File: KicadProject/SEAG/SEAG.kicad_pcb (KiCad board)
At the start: 4 copper layers, 99.6 x 63 mm, 64 parts, among them J1 Screw_Terminal_01x02, J10 Screw_Terminal_01x02, J11 Screw_Terminal_01x02, J12 Screw_Terminal_01x02, J13 Conn_01x03_Pin, J2 Conn_01x06_Pin, J3 Screw_Terminal_01x02, J4 Screw_Terminal_01x02, J5 Screw_Terminal_01x02, J6 Screw_Terminal_01x02, J7 Screw_Terminal_01x02, J8 Screw_Terminal_01x02, J9 Screw_Terminal_01x02, U1 STM32F722RCTx, X1 XO32, Y1 Crystal_GND24

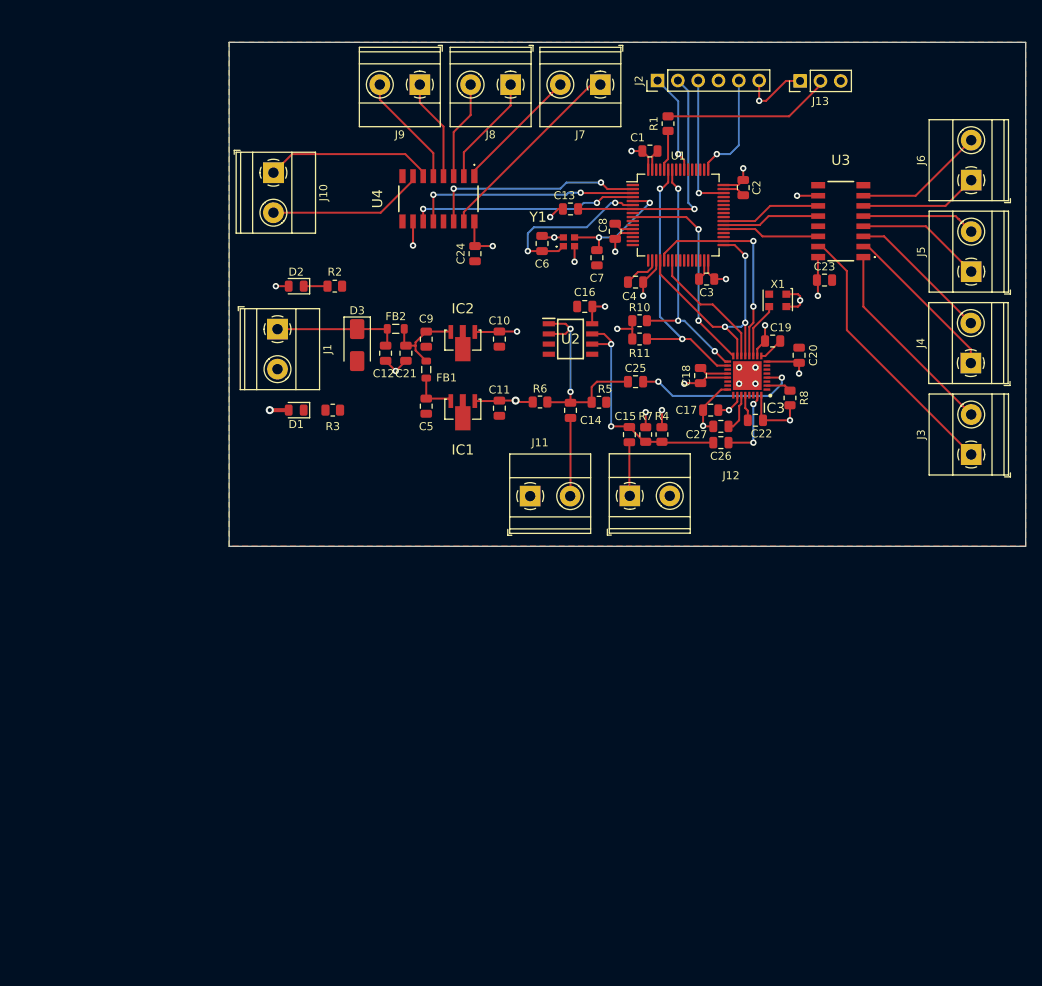
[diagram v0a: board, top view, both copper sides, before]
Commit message: PCB rev 2
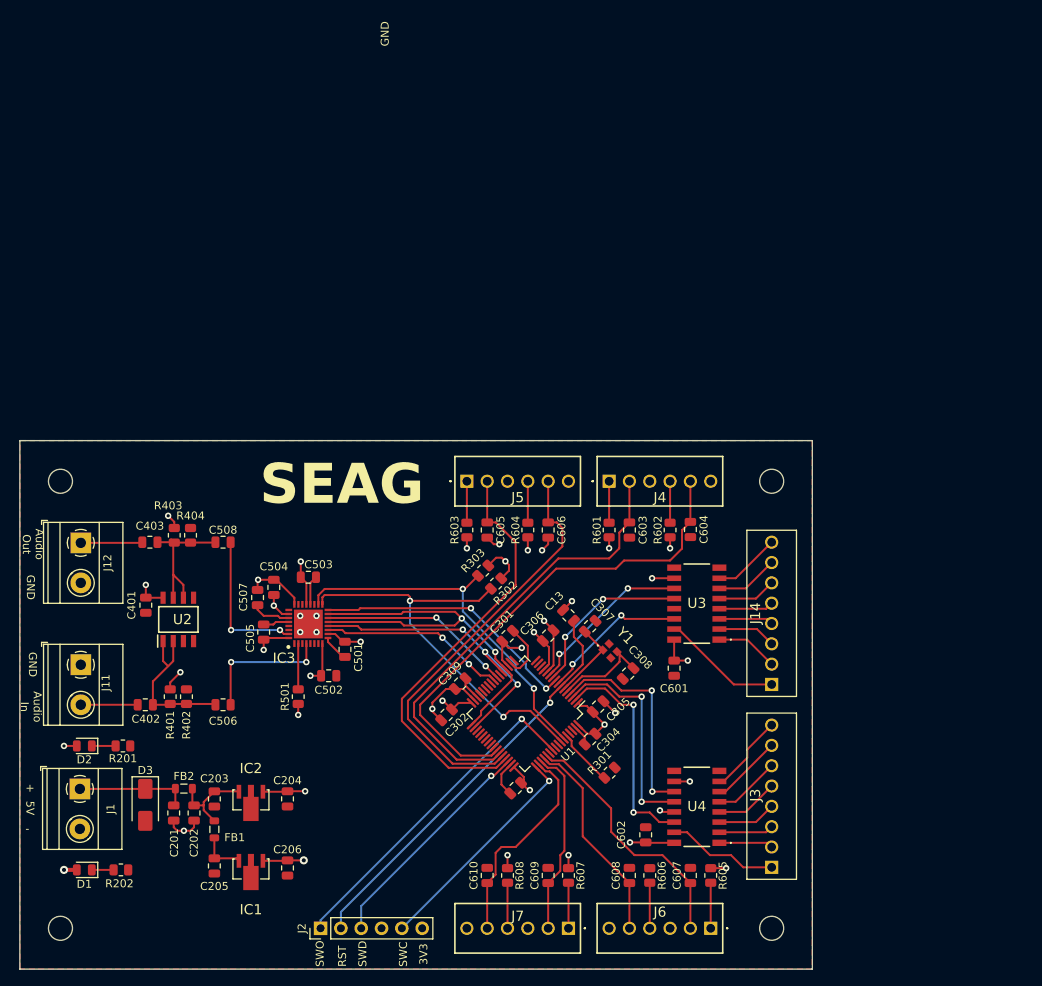
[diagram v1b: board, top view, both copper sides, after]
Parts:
- removed J10, J8, J9: Screw_Terminal_01x02, TerminalBlock_Phoenix:TerminalBlock_Phoenix_MKDS-1,5-2_1x02_P5.00mm_Horizontal
- removed J13: Conn_01x03_Pin, Connector_PinHeader_2.54mm:PinHeader_1x03_P2.54mm_Vertical
- removed R8: 33k, Resistor_SMD:R_0805_2012Metric
- removed X1: XO32, Oscillator:Oscillator_SMD_EuroQuartz_XO32-4Pin_3.2x2.5mm
- added C305: 100n, Capacitor_SMD:C_0805_2012Metric, F.Cu at (123.1, 119.6)
- added C309: 4.7u, Capacitor_SMD:C_0805_2012Metric, F.Cu at (105.8, 116.7)
- added C603: 100n, Capacitor_SMD:C_0805_2012Metric, F.Cu at (127.0, 97.5)
- added C604: 100n, Capacitor_SMD:C_0805_2012Metric, F.Cu at (134.6, 97.5)
- added C605: 100n, Capacitor_SMD:C_0805_2012Metric, F.Cu at (109.2, 97.5)
- added C606: 100n, Capacitor_SMD:C_0805_2012Metric, F.Cu at (116.8, 97.5)
- added C607: 100n, Capacitor_SMD:C_0805_2012Metric, F.Cu at (134.6, 140.7)
- added C608: 100n, Capacitor_SMD:C_0805_2012Metric, F.Cu at (127.0, 140.7)
- added C609: 100n, Capacitor_SMD:C_0805_2012Metric, F.Cu at (116.8, 140.7)
- added C610: 100n, Capacitor_SMD:C_0805_2012Metric, F.Cu at (109.2, 140.7)
- added H1: MountingHole, MountingHole:MountingHole_3mm, F.Cu at (55.9, 91.4)
- added H2: MountingHole, MountingHole:MountingHole_3mm, F.Cu at (55.9, 147.3)
- added H3: MountingHole, MountingHole:MountingHole_3mm, F.Cu at (144.8, 91.4)
- added H4: MountingHole, MountingHole:MountingHole_3mm, F.Cu at (144.8, 147.3)
- added J14: Screw_Terminal_01x08, SamacSys_Parts:1725711, F.Cu at (144.8, 116.8)
- added R501: 33k, Resistor_SMD:R_0805_2012Metric, F.Cu at (85.6, 118.4)
- added R601: 10K, Resistor_SMD:R_0805_2012Metric, F.Cu at (124.5, 97.5)
- added R602: 10K, Resistor_SMD:R_0805_2012Metric, F.Cu at (132.1, 97.5)
- added R603: 10K, Resistor_SMD:R_0805_2012Metric, F.Cu at (106.7, 97.5)
- added R604: 10K, Resistor_SMD:R_0805_2012Metric, F.Cu at (114.3, 97.5)
- added R605: 10K, Resistor_SMD:R_0805_2012Metric, F.Cu at (137.2, 140.7)
- added R606: 10K, Resistor_SMD:R_0805_2012Metric, F.Cu at (129.5, 140.7)
- added R607: 10K, Resistor_SMD:R_0805_2012Metric, F.Cu at (119.4, 140.7)
- added R608: 10K, Resistor_SMD:R_0805_2012Metric, F.Cu at (111.8, 140.7)
- J3: value Screw_Terminal_01x02 -> Screw_Terminal_01x08; footprint TerminalBlock_Phoenix:TerminalBlock_Phoenix_MKDS-1,5-2_1x02_P5.00mm_Horizontal -> SamacSys_Parts:1725711
- J4, J5, J6, J7: value Screw_Terminal_01x02 -> Screw_Terminal_01x06; footprint TerminalBlock_Phoenix:TerminalBlock_Phoenix_MKDS-1,5-2_1x02_P5.00mm_Horizontal -> SamacSys_Parts:1725698
- moved J2 114.0 mm to (88.4, 147.3)
- moved J7 105.5 mm to (119.4, 147.3)
- moved J6 99.0 mm to (137.2, 147.3), turned to 180 degrees
- moved U4 82.6 mm to (135.4, 132.1), turned to 180 degrees
- moved R301 81.5 mm to (124.5, 127.9), turned to -135 degrees
- moved C303 80.3 mm to (112.8, 129.8), turned to -135 degrees
- moved C602 75.7 mm to (129.0, 135.6), turned to 90 degrees
- moved C304 73.9 mm to (122.1, 123.7), turned to -135 degrees
- moved C502 71.1 mm to (89.4, 115.8), turned to 0 degrees
- moved J12 68.9 mm to (58.4, 99.1), turned to -90 degrees
- moved J5 68.3 mm to (106.7, 91.4), turned to 0 degrees
- moved C505 66.9 mm to (81.3, 110.3), turned to 90 degrees
- moved C401 66.4 mm to (66.5, 106.9), turned to -90 degrees
- moved C501 65.9 mm to (91.4, 112.5), turned to -90 degrees
- moved C506 65.5 mm to (76.2, 119.4)
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- renumbered C12 to C201, C21 to C202, C9 to C203, C10 to C204, C5 to C205, C11 to C206, C4 to C301, C3 to C302, C2 to C303, C1 to C304, C8 to C306, C6 to C307, C7 to C308, C16 to C401, C14 to C402, C15 to C403, C19 to C501, C20 to C502, C18 to C503, C17 to C504, C22 to C505, C25 to C506, C27 to C507, C26 to C508, C23 to C601, C24 to C602, R2 to R201, R3 to R202, R1 to R301, R10 to R302, R11 to R303, R6 to R401, R5 to R402, R4 to R403, R7 to R404
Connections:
- IC3 pad 11: /Codec/OscOut -> MCLK
- J3 pad 1: /IO/Q0b -> /IO/Q0l
- J3 pad 2: /IO/Q1b -> /IO/Q1l
- J4 pad 1: /IO/Q2b -> Net-(J4-Pin_1)
- J4 pad 2: /IO/Q3b -> ToggleInput1
- J5 pad 1: /IO/Q4b -> Net-(J5-Pin_1)
- J5 pad 2: /IO/Q5b -> ToggleInput3
- J6 pad 1: /IO/Q6b -> Net-(J6-Pin_1)
- J6 pad 2: /IO/Q7b -> ToggleInput5
- J7 pad 1: /IO/Q0l -> Net-(J7-Pin_1)
- J7 pad 2: /IO/Q1l -> ToggleInput7
- R202 pad 1: GND -> Net-(D1-K)
- R202 pad 2: Net-(D1-K) -> GND
- R301 pad 1: Net-(J13-Pin_2) -> GND
- U1 pad 10: unconnected-(U1-PC2-Pad10) -> ShiftRegBarClk
- U1 pad 11: unconnected-(U1-PC3-Pad11) -> ShiftRegBarStoClk
- U1 pad 24: unconnected-(U1-PC4-Pad24) -> MCLK
- U1 pad 30: unconnected-(U1-VCAP_1-Pad30) -> Net-(U1-VCAP_1)
- U1 pad 37: ShiftRegBarDat -> unconnected-(U1-PC6-Pad37)
- U1 pad 38: ShiftRegBarClk -> unconnected-(U1-PC7-Pad38)
- U1 pad 39: ShiftRegBarStoClk -> unconnected-(U1-PC8-Pad39)
- U1 pad 42: unconnected-(U1-PA9-Pad42) -> ToggleInput2
- U1 pad 43: unconnected-(U1-PA10-Pad43) -> ToggleInput1
- U1 pad 44: unconnected-(U1-PA11-Pad44) -> ToggleInput4
- U1 pad 45: unconnected-(U1-PA12-Pad45) -> ToggleInput3
- U1 pad 50: unconnected-(U1-PA15-Pad50) -> ToggleInput8
- U1 pad 51: unconnected-(U1-PC10-Pad51) -> ToggleInput7
- U1 pad 52: unconnected-(U1-PC11-Pad52) -> ToggleInput6
- U1 pad 53: unconnected-(U1-PC12-Pad53) -> ToggleInput5
- U1 pad 8: unconnected-(U1-PC0-Pad8) -> ShiftRegBarDat
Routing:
- net ToggleInput2: track 0.00 -> 63.0 mm
- net ToggleInput1: track 0.00 -> 57.6 mm
- net ToggleInput3: track 0.00 -> 53.8 mm
- net ToggleInput4: track 0.00 -> 53.6 mm
- net +3.3VA: track 127.6 -> 175.4 mm, vias 8 -> 10
- net ToggleInput5: track 0.00 -> 31.9 mm
- net /MCU/SWO: track 12.5 -> 42.1 mm
- net ToggleInput8: track 0.00 -> 26.5 mm
- net ToggleInput6: track 0.00 -> 26.3 mm
- net ToggleInput7: track 0.00 -> 23.5 mm
- net MCLK: track 0.00 -> 23.4 mm, vias 0 -> 2
- net Net-(J13-Pin_2): track 21.2 -> 0.00 mm
- net I2C.SCL: track 31.4 -> 52.1 mm, vias 3 -> 2
- net /MCU/NRST: track 31.5 -> 51.7 mm
- net /IO/Q0b: track 34.2 -> 15.1 mm
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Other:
- board size 99.6 x 63 mm -> 99.1 x 66.1 mm
- board text added: "+"
- board text added: "-"
- board text added: "3V3"
- board text added: "5V"
- board text added: "Audio In"
- board text added: "Audio Out"
- board text added: "GND"
- board text added: "RST"
- board text added: "SEAG"
- board text added: "SWC"
- board text added: "SWD"
- board text added: "SWO"
